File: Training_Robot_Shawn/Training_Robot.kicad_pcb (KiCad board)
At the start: 2 copper layers, 87.1 x 87 mm, 16 parts, among them J1 Arduino connector, J4 3v3, J5 GND, M1 FrontL, M2 FrontR, M3 BackL, M4 BackR, SW1 SW_SPDT_312

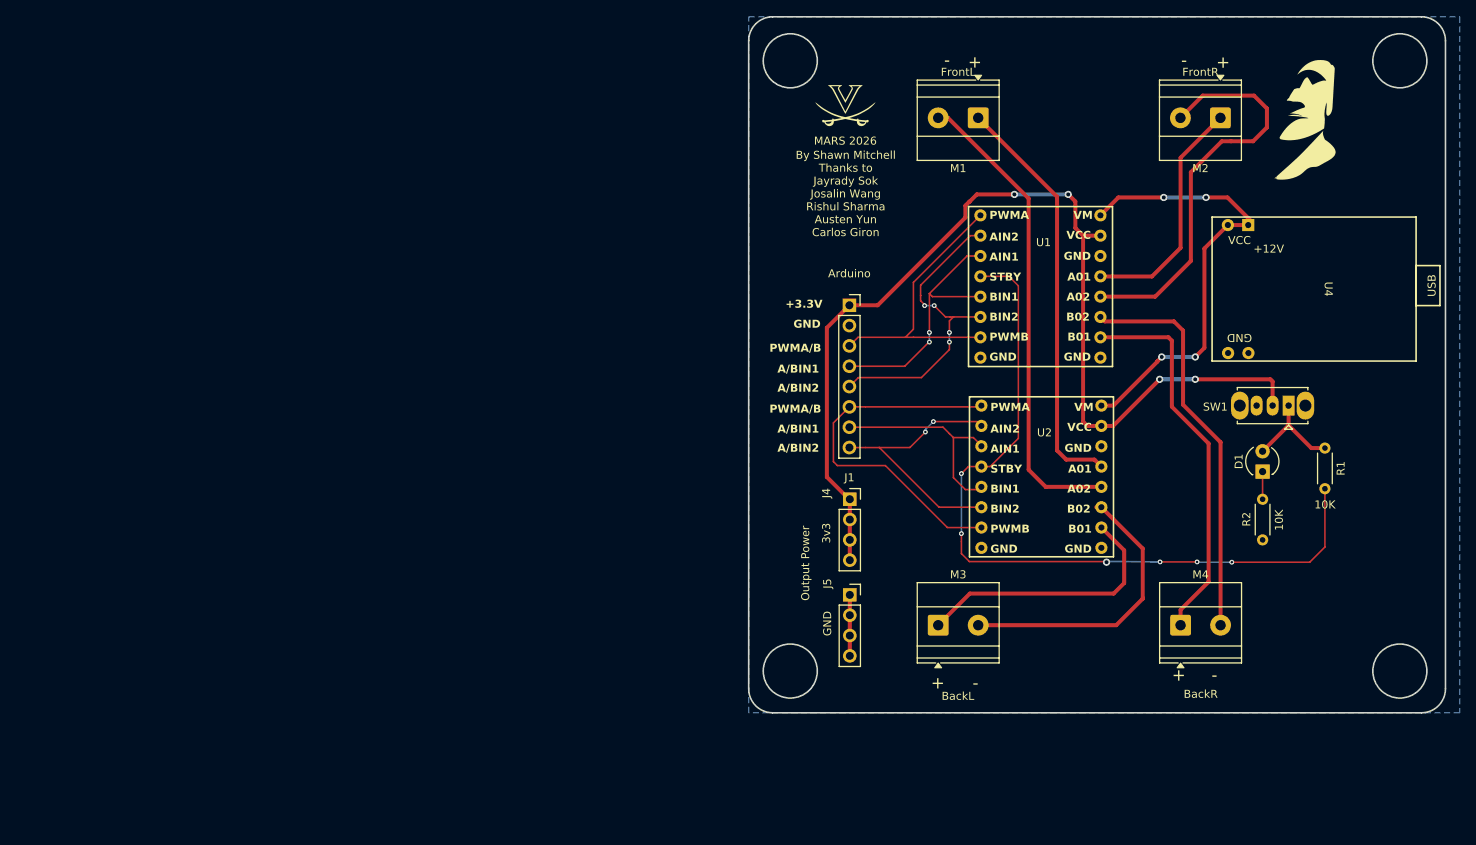
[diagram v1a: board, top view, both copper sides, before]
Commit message: first revision of layout
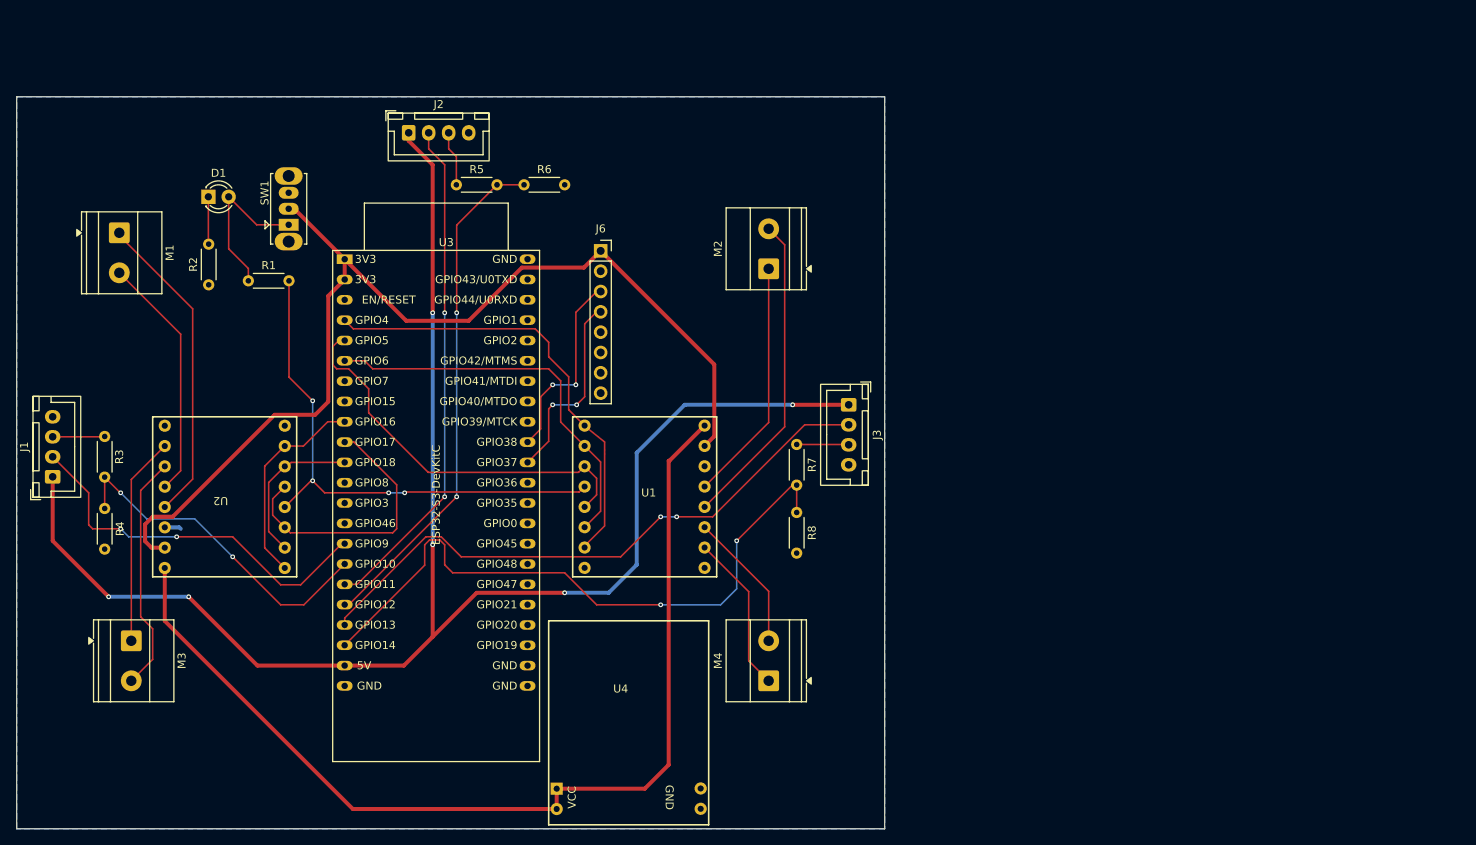
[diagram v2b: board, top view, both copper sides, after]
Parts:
- removed G***: LOGO, Library:Moai4
- removed G***: LOGO, Library:UVA_logo_new
- removed J4: 3v3, Connector_PinSocket_2.54mm:PinSocket_1x04_P2.54mm_Vertical
- removed J5: GND, Connector_PinSocket_2.54mm:PinSocket_1x04_P2.54mm_Vertical
- added J2: Conn_01x04_Pin, Connector_JST:JST_XH_B4B-XH-A_1x04_P2.50mm_Vertical, F.Cu at (92.0, 43.5)
- added J3: Conn_01x04_Pin, Connector_JST:JST_XH_B4B-XH-A_1x04_P2.50mm_Vertical, F.Cu at (147.0, 77.5)
- added J6: Conn_01x08_Socket, Connector_PinSocket_2.54mm:PinSocket_1x08_P2.54mm_Vertical, F.Cu at (116.0, 58.3)
- added R3: 1k, Resistor_THT:R_Axial_DIN0204_L3.6mm_D1.6mm_P5.08mm_Horizontal, F.Cu at (54.0, 81.5)
- added R4: 2k, Resistor_THT:R_Axial_DIN0204_L3.6mm_D1.6mm_P5.08mm_Horizontal, F.Cu at (54.0, 90.5)
- added R5: 1k, Resistor_THT:R_Axial_DIN0204_L3.6mm_D1.6mm_P5.08mm_Horizontal, F.Cu at (98.0, 50.0)
- added R6: 2k, Resistor_THT:R_Axial_DIN0204_L3.6mm_D1.6mm_P5.08mm_Horizontal, F.Cu at (106.4, 50.0)
- added R7: 1k, Resistor_THT:R_Axial_DIN0204_L3.6mm_D1.6mm_P5.08mm_Horizontal, F.Cu at (140.5, 82.5)
- added R8: 2k, Resistor_THT:R_Axial_DIN0204_L3.6mm_D1.6mm_P5.08mm_Horizontal, F.Cu at (140.5, 91.0)
- added U3: ESP32-S3-DevKitC, PCM_Espressif:ESP32-S3-DevKitC, F.Cu at (84.0, 59.3)
- J1: value Arduino connector -> Conn_01x04_Pin; footprint Connector_PinSocket_2.54mm:PinSocket_1x08_P2.54mm_Vertical -> Connector_JST:JST_XH_B4B-XH-A_1x04_P2.50mm_Vertical
- U1, U2: footprint Library:TB_breakout_motor_driver -> MARS Custom Footprints:TB6612FNG Breakout
- U4: footprint Library:PD Module -> MARS Custom Footprints:USB PD Module
- moved R1 136.2 mm to (72.0, 62.0), turned to 0 degrees
- moved D1 136.2 mm to (67.0, 51.5), turned to 0 degrees
- moved R2 135.5 mm to (67.0, 62.5)
- moved SW1 127.0 mm to (77.0, 55.0), turned to 90 degrees
- moved M1 108.3 mm to (55.8, 56.0), turned to -90 degrees
- moved U4 104.4 mm to (118.5, 113.5), turned to 0 degrees
- moved U2 102.9 mm to (68.5, 89.0), turned to 180 degrees
- moved J1 101.9 mm to (47.5, 86.5), turned to 90 degrees
- moved M3 100.9 mm to (57.3, 107.0), turned to -90 degrees
- moved M2 59.5 mm to (137.0, 60.5), turned to 90 degrees
- moved U1 57.6 mm to (122.0, 89.0)
- moved M4 52.0 mm to (137.0, 112.0), turned to 90 degrees
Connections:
- net +12V motor pwr renamed +12V
- J1 pad 1: +3V3 -> +5V
- J1 pad 2: GND -> /L_US_TRIG
- J1 pad 4: Net-(J1-Pin_4) -> GND
- U1 pad 1: Net-(J1-Pin_3) -> /RIGHT_EN
- U1 pad 2: Net-(J1-Pin_5) -> /RIGHT_BACKWARD
- U1 pad 3: Net-(J1-Pin_4) -> /RIGHT_FORWARD
- U1 pad 5: Net-(J1-Pin_4) -> /RIGHT_FORWARD
- U1 pad 6: Net-(J1-Pin_5) -> /RIGHT_BACKWARD
- U1 pad 7: Net-(J1-Pin_3) -> /RIGHT_EN
- U2 pad 1: Net-(J1-Pin_6) -> /LEFT_EN
- U2 pad 2: Net-(J1-Pin_8) -> /LEFT_BACKWARD
- U2 pad 3: Net-(J1-Pin_7) -> /LEFT_FORWARD
- U2 pad 5: Net-(J1-Pin_7) -> /LEFT_FORWARD
- U2 pad 6: Net-(J1-Pin_8) -> /LEFT_BACKWARD
- U2 pad 7: Net-(J1-Pin_6) -> /LEFT_EN
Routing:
- net +5V: track 0.00 -> 199.9 mm, vias 0 -> 6
- net /R_US_ECHO: track 0.00 -> 81.4 mm, vias 0 -> 2
- net /R_US_TRIG: track 0.00 -> 75.9 mm, vias 0 -> 2
- net +12V: track 56.7 -> 127.4 mm, vias 4 -> 0
- net /F_US_ECHO: track 0.00 -> 64.1 mm, vias 0 -> 2
- net /F_US_TRIG: track 0.00 -> 63.4 mm, vias 0 -> 2
- net /RIGHT_FORWARD: track 0.00 -> 49.5 mm
- net /RIGHT_BACKWARD: track 0.00 -> 49.2 mm
- net /L_US_TRIG: track 0.00 -> 47.6 mm, vias 0 -> 2
- net Net-(J1-Pin_6): track 46.1 -> 0.00 mm
- net /L_US_ECHO: track 0.00 -> 42.6 mm, vias 0 -> 2
- net Net-(J1-Pin_5): track 39.1 -> 0.00 mm, vias 4 -> 0
- net /RIGHT_EN: track 0.00 -> 39.0 mm
- net /LEFT_FORWARD: track 0.00 -> 35.0 mm
- net Net-(J1-Pin_8): track 34.3 -> 0.00 mm, vias 2 -> 0
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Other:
- board size 87.1 x 87 mm -> 108.5 x 91.5 mm
- board text removed: "+"
- board text removed: "+12V"
- board text removed: "+3.3V"
- board text removed: "-"
- board text removed: "10K"
- board text removed: "A/BIN1"
- board text removed: "A/BIN2"
- board text removed: "A01"
- board text removed: "A02"
- board text removed: "AIN1"
- board text removed: "AIN2"
- board text removed: "Arduino"
- board text removed: "B01"
- board text removed: "B02"
- board text removed: "BIN1"
- board text removed: "BIN2"
- board text removed: "By Shawn Mitchell Thanks to Jayrady Sok Josalin Wang Rishul Sharma Austen Yun Carlos Giron"
- board text removed: "GND"
- board text removed: "J1"
- board text removed: "MARS 2026"
- board text removed: "Output Power"
- board text removed: "PWMA"
- board text removed: "PWMA/B"
- board text removed: "PWMB"
- board text removed: "STBY"
- board text removed: "USB"
- board text removed: "VCC"
- board text removed: "VM"
